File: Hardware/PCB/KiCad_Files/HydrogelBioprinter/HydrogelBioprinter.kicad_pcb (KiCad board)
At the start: 2 copper layers, 50 parts, among them Q10 MMBT4403_, Q5 RFP30N06LE, Q7 RFP30N06LE, Q8 RFP30N06LE, Q9 RFP30N06LE, U1 STM32F407VGT6, U2 M24C64-WMN6TP, U3 LM5116MHX_NOPB, U5 MAX6675ISA_, U6 TMUX1208PWR, U7 SN74HC245DWR, U9 HX711

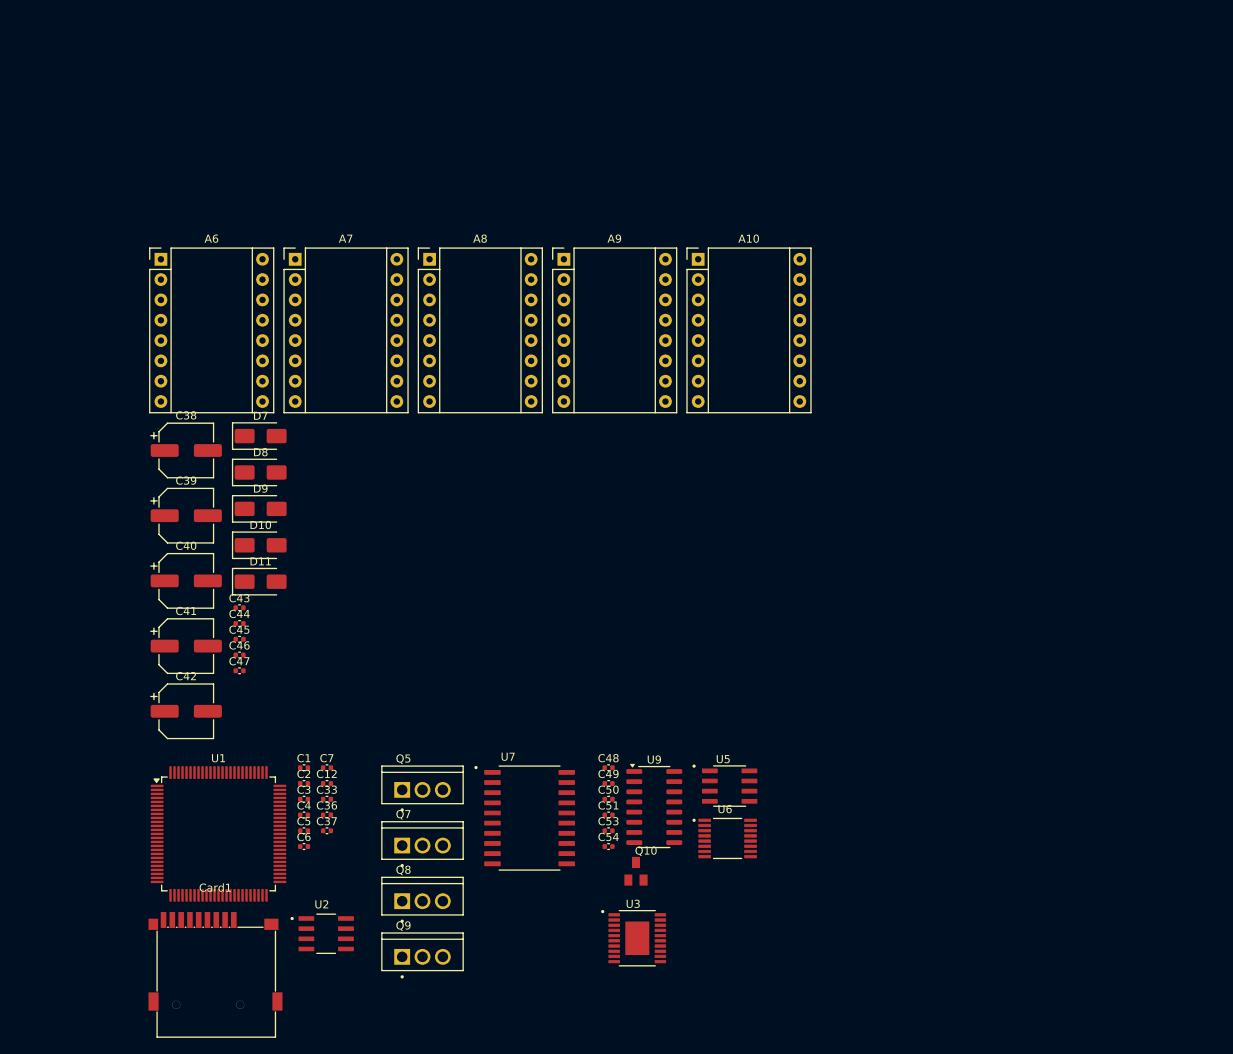
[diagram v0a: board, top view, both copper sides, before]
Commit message: Schematic Update, PCB preliminary layout, Machine Design addition, and LaTeX report addition
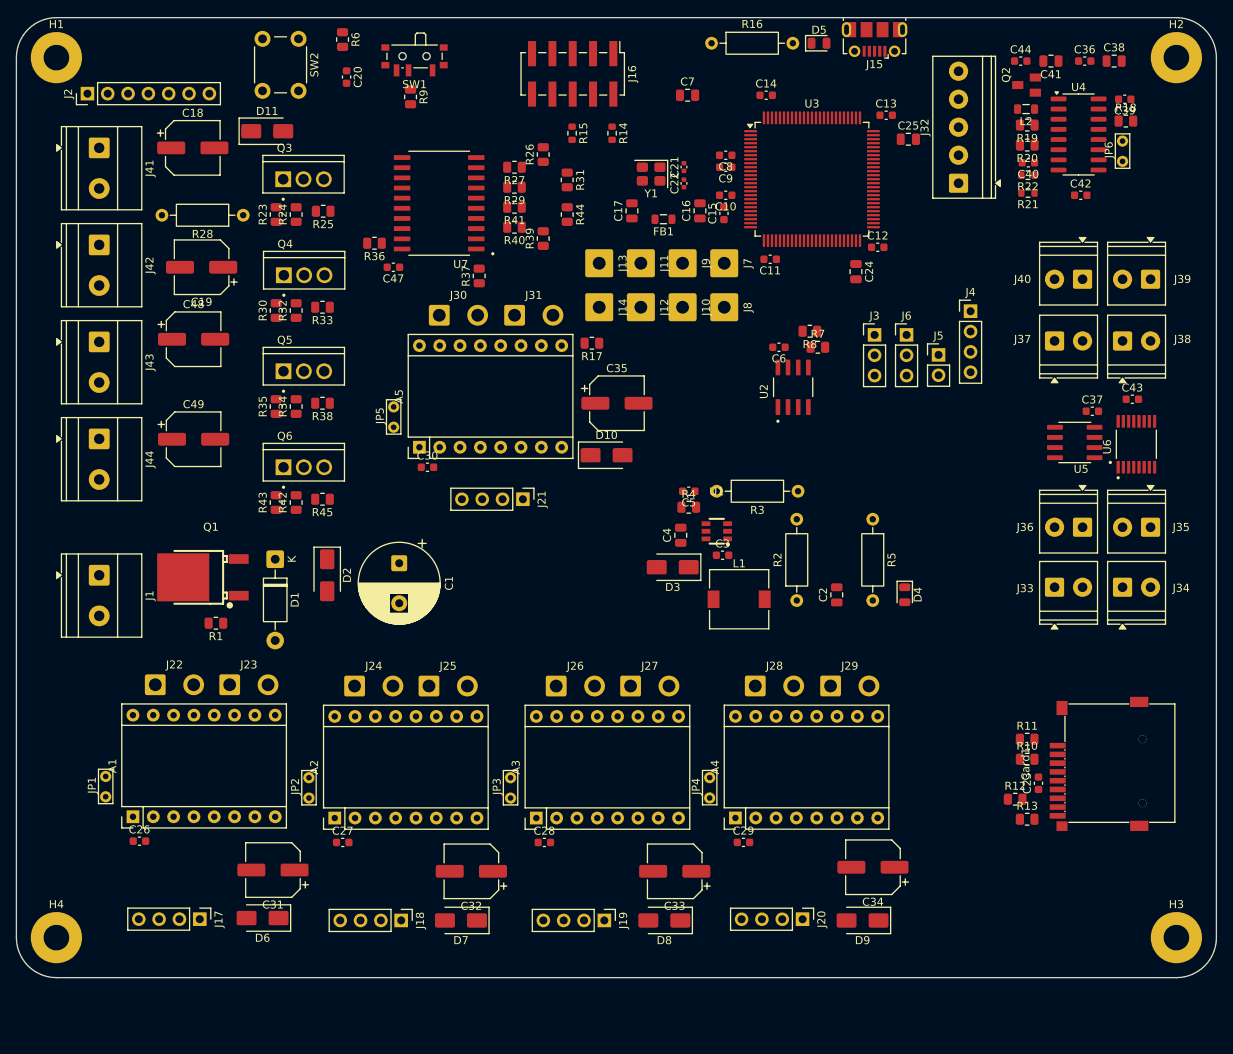
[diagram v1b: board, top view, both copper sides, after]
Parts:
- removed A10, A6, A7, A8, A9: MKS TMC2209, Module:Pololu_Breakout-16_15.2x20.3mm
- removed C45, C46, C50, C51, C53, C54: 100n, Capacitor_SMD:C_0402_1005Metric
- removed Q10: MMBT4403_, MMBT4403_:SOT23-BEC
- removed Q7, Q8, Q9: RFP30N06LE, RFP30N06LE:TRANS_RFP30N06LE
- removed U9: HX711, Package_SO:SOP-16_3.9x9.9mm_P1.27mm
- added A1: MKS TMC2209, Module:Pololu_Breakout-16_15.2x20.3mm, F.Cu at (82.6, 132.4)
- added A2: MKS TMC2209, Module:Pololu_Breakout-16_15.2x20.3mm, F.Cu at (107.8, 132.6)
- added A3: MKS TMC2209, Module:Pololu_Breakout-16_15.2x20.3mm, F.Cu at (133.0, 132.6)
- added A4: MKS TMC2209, Module:Pololu_Breakout-16_15.2x20.3mm, F.Cu at (157.9, 132.5)
- added A5: MKS TMC2209, Module:Pololu_Breakout-16_15.2x20.3mm, F.Cu at (118.4, 86.2)
- added C10: 100n, Capacitor_SMD:C_0603_1608Metric, F.Cu at (156.7, 54.7)
- added C11: 100n, Capacitor_SMD:C_0603_1608Metric, F.Cu at (162.2, 62.7)
- added C13: 100n, Capacitor_SMD:C_0603_1608Metric, F.Cu at (176.7, 44.7)
- added C14: 100n, Capacitor_SMD:C_0603_1608Metric, F.Cu at (161.7, 42.2)
- added C15: 10n, Capacitor_SMD:C_0603_1608Metric, F.Cu at (156.4, 57.0)
- added C16: 1u, Capacitor_SMD:C_0805_2012Metric, F.Cu at (153.4, 56.6)
- added C17: 1u, Capacitor_SMD:C_0805_2012Metric, F.Cu at (144.9, 56.6)
- added C18: 100u, Capacitor_SMD:CP_Elec_6.3x7.7, F.Cu at (90.0, 48.8)
- added C19: 100u, Capacitor_SMD:CP_Elec_6.3x7.7, F.Cu at (91.2, 63.7)
- added C20: 100n, Capacitor_SMD:C_0603_1608Metric, F.Cu at (109.3, 39.9)
- added C21: 10p, Capacitor_SMD:C_0402_1005Metric, F.Cu at (151.4, 51.2)
- added C22: 10p, Capacitor_SMD:C_0402_1005Metric, F.Cu at (151.4, 53.2)
- added C23: 100n, Capacitor_SMD:C_0603_1608Metric, F.Cu at (195.8, 128.2)
- added C24: 2.2uF, Capacitor_SMD:C_0805_2012Metric, F.Cu at (172.9, 64.2)
- added C25: 2.2uF, Capacitor_SMD:C_0805_2012Metric, F.Cu at (179.5, 47.7)
- added C26: 100n, Capacitor_SMD:C_0603_1608Metric, F.Cu at (83.4, 135.4)
- added C27: 100n, Capacitor_SMD:C_0603_1608Metric, F.Cu at (108.8, 135.6)
- added C28: 100n, Capacitor_SMD:C_0603_1608Metric, F.Cu at (134.0, 135.6)
- added C29: 100n, Capacitor_SMD:C_0603_1608Metric, F.Cu at (158.9, 135.6)
- added C30: 100n, Capacitor_SMD:C_0603_1608Metric, F.Cu at (119.4, 88.7)
- added C31: 100u, Capacitor_SMD:CP_Elec_6.3x7.7, F.Cu at (100.1, 139.1)
- added C32: 100u, Capacitor_SMD:CP_Elec_6.3x7.7, F.Cu at (124.9, 139.2)
- added C34: 100u, Capacitor_SMD:CP_Elec_6.3x7.7, F.Cu at (175.1, 138.7)
- added C35: 100u, Capacitor_SMD:CP_Elec_6.3x7.7, F.Cu at (143.1, 80.7)
- added C8: 100n, Capacitor_SMD:C_0603_1608Metric, F.Cu at (156.7, 49.7)
- added C9: 100n, Capacitor_SMD:C_0603_1608Metric, F.Cu at (156.7, 51.2)
- added D1: 1N4744A, Diode_THT:D_DO-41_SOD81_P10.16mm_Horizontal, F.Cu at (100.3, 100.2)
- added D2: SMAJ16A, Diode_SMD:D_SMA, F.Cu at (106.8, 102.2)
- added D3: SS34, Diode_SMD:D_SMA, F.Cu at (150.0, 101.2)
- added D4: GREEN, LED_SMD:LED_0805_2012Metric, F.Cu at (179.0, 104.6)
- added D5: BLUE, LED_SMD:LED_0805_2012Metric, F.Cu at (168.3, 35.7)
- added D6: SMAJ16A, Diode_SMD:D_SMA, F.Cu at (98.8, 145.1)
- added FB1: 120R, Inductor_SMD:L_0805_2012Metric, F.Cu at (148.9, 57.7)
- added H1: MountingHole_Pad, MountingHole:MountingHole_3.2mm_M3_Pad, F.Cu at (73.0, 37.5)
- added H2: MountingHole_Pad, MountingHole:MountingHole_3.2mm_M3_Pad, F.Cu at (213.0, 37.5)
- added H3: MountingHole_Pad, MountingHole:MountingHole_3.2mm_M3_Pad, F.Cu at (213.0, 147.5)
- added H4: MountingHole_Pad, MountingHole:MountingHole_3.2mm_M3_Pad, F.Cu at (73.0, 147.5)
- added J1: Screw_Terminal_01x02, TerminalBlock_Phoenix:TerminalBlock_Phoenix_MKDS-1,5-2-5.08_1x02_P5.08mm_Horizontal, F.Cu at (78.3, 102.2)
- added J10: Conn, Connector_Wire:SolderWire-0.75sqmm_1x01_D1.25mm_OD3.5mm, F.Cu at (151.3, 68.7)
- added J11: Conn, Connector_Wire:SolderWire-0.75sqmm_1x01_D1.25mm_OD3.5mm, F.Cu at (146.1, 63.2)
- added J12: Conn, Connector_Wire:SolderWire-0.75sqmm_1x01_D1.25mm_OD3.5mm, F.Cu at (146.1, 68.7)
- added J13: Conn, Connector_Wire:SolderWire-0.75sqmm_1x01_D1.25mm_OD3.5mm, F.Cu at (140.8, 63.2)
- added J14: Conn, Connector_Wire:SolderWire-0.75sqmm_1x01_D1.25mm_OD3.5mm, F.Cu at (140.8, 68.7)
- added J15: USB_B_Micro, Connector_USB:USB_Micro-B_Molex-105017-0001, F.Cu at (175.3, 35.2)
- added J16: Conn_02x05_Odd_Even, Connector_PinHeader_2.54mm:PinHeader_2x05_P2.54mm_Vertical_SMD, F.Cu at (137.5, 39.5)
- added J17: Conn_01x04_Pin, Connector_PinHeader_2.54mm:PinHeader_1x04_P2.54mm_Vertical, F.Cu at (90.9, 145.2)
- added J18: Conn_01x04_Pin, Connector_PinHeader_2.54mm:PinHeader_1x04_P2.54mm_Vertical, F.Cu at (116.1, 145.3)
- added J19: Conn_01x04_Pin, Connector_PinHeader_2.54mm:PinHeader_1x04_P2.54mm_Vertical, F.Cu at (141.5, 145.3)
- added J2: Conn_01x07_Pin, Connector_PinHeader_2.54mm:PinHeader_1x07_P2.54mm_Vertical, F.Cu at (76.9, 42.0)
- added J20: Conn_01x04_Pin, Connector_PinHeader_2.54mm:PinHeader_1x04_P2.54mm_Vertical, F.Cu at (166.3, 145.2)
- added J21: Conn_01x04_Pin, Connector_PinHeader_2.54mm:PinHeader_1x04_P2.54mm_Vertical, F.Cu at (131.3, 92.7)
- added J22: Conn, Connector_Wire:SolderWire-0.75sqmm_1x02_P4.8mm_D1.25mm_OD2.3mm, F.Cu at (85.4, 115.9)
- added J23: Conn, Connector_Wire:SolderWire-0.75sqmm_1x02_P4.8mm_D1.25mm_OD2.3mm, F.Cu at (94.7, 115.9)
- added J24: Conn, Connector_Wire:SolderWire-0.75sqmm_1x02_P4.8mm_D1.25mm_OD2.3mm, F.Cu at (110.3, 116.0)
- added J25: Conn, Connector_Wire:SolderWire-0.75sqmm_1x02_P4.8mm_D1.25mm_OD2.3mm, F.Cu at (119.6, 116.0)
- added J26: Conn, Connector_Wire:SolderWire-0.75sqmm_1x02_P4.8mm_D1.25mm_OD2.3mm, F.Cu at (135.5, 116.0)
- added J27: Conn, Connector_Wire:SolderWire-0.75sqmm_1x02_P4.8mm_D1.25mm_OD2.3mm, F.Cu at (144.8, 116.0)
- added J28: Conn, Connector_Wire:SolderWire-0.75sqmm_1x02_P4.8mm_D1.25mm_OD2.3mm, F.Cu at (160.4, 116.0)
- added J29: Conn, Connector_Wire:SolderWire-0.75sqmm_1x02_P4.8mm_D1.25mm_OD2.3mm, F.Cu at (169.8, 116.0)
- added J3: Conn_01x03_Pin, Connector_PinHeader_2.54mm:PinHeader_1x03_P2.54mm_Vertical, F.Cu at (175.3, 72.2)
- added J30: Conn, Connector_Wire:SolderWire-0.75sqmm_1x02_P4.8mm_D1.25mm_OD2.3mm, F.Cu at (120.9, 69.7)
- added J31: Conn, Connector_Wire:SolderWire-0.75sqmm_1x02_P4.8mm_D1.25mm_OD2.3mm, F.Cu at (130.3, 69.7)
- added J32: Screw_Terminal_01x05, TerminalBlock_Phoenix:TerminalBlock_Phoenix_PT-1,5-5-3.5-H_1x05_P3.50mm_Horizontal, F.Cu at (185.8, 53.2)
- added J33: Screw_Terminal_01x02, TerminalBlock_Phoenix:TerminalBlock_Phoenix_PT-1,5-2-3.5-H_1x02_P3.50mm_Horizontal, F.Cu at (197.8, 103.7)
- added J34: Screw_Terminal_01x02, TerminalBlock_Phoenix:TerminalBlock_Phoenix_PT-1,5-2-3.5-H_1x02_P3.50mm_Horizontal, F.Cu at (206.3, 103.7)
- added J35: Screw_Terminal_01x02, TerminalBlock_Phoenix:TerminalBlock_Phoenix_PT-1,5-2-3.5-H_1x02_P3.50mm_Horizontal, F.Cu at (209.8, 96.2)
- added J36: Screw_Terminal_01x02, TerminalBlock_Phoenix:TerminalBlock_Phoenix_PT-1,5-2-3.5-H_1x02_P3.50mm_Horizontal, F.Cu at (201.3, 96.2)
- added J37: Screw_Terminal_01x02, TerminalBlock_Phoenix:TerminalBlock_Phoenix_PT-1,5-2-3.5-H_1x02_P3.50mm_Horizontal, F.Cu at (197.8, 72.9)
- added J38: Screw_Terminal_01x02, TerminalBlock_Phoenix:TerminalBlock_Phoenix_PT-1,5-2-3.5-H_1x02_P3.50mm_Horizontal, F.Cu at (206.3, 72.9)
- added J39: Screw_Terminal_01x02, TerminalBlock_Phoenix:TerminalBlock_Phoenix_PT-1,5-2-3.5-H_1x02_P3.50mm_Horizontal, F.Cu at (209.8, 65.2)
- added J4: Conn_01x04_Pin, Connector_PinHeader_2.54mm:PinHeader_1x04_P2.54mm_Vertical, F.Cu at (187.3, 69.2)
- added J40: Screw_Terminal_01x02, TerminalBlock_Phoenix:TerminalBlock_Phoenix_PT-1,5-2-3.5-H_1x02_P3.50mm_Horizontal, F.Cu at (201.3, 65.2)
- added J41: Screw_Terminal_01x02, TerminalBlock_Phoenix:TerminalBlock_Phoenix_MKDS-1,5-2-5.08_1x02_P5.08mm_Horizontal, F.Cu at (78.3, 48.8)
- added J42: Screw_Terminal_01x02, TerminalBlock_Phoenix:TerminalBlock_Phoenix_MKDS-1,5-2-5.08_1x02_P5.08mm_Horizontal, F.Cu at (78.3, 60.9)
- added J43: Screw_Terminal_01x02, TerminalBlock_Phoenix:TerminalBlock_Phoenix_MKDS-1,5-2-5.08_1x02_P5.08mm_Horizontal, F.Cu at (78.3, 73.0)
- added J44: Screw_Terminal_01x02, TerminalBlock_Phoenix:TerminalBlock_Phoenix_MKDS-1,5-2-5.08_1x02_P5.08mm_Horizontal, F.Cu at (78.3, 85.2)
- added J5: Conn_01x02_Pin, Connector_PinHeader_2.54mm:PinHeader_1x02_P2.54mm_Vertical, F.Cu at (183.3, 74.7)
- added J6: Conn_01x03_Pin, Connector_PinHeader_2.54mm:PinHeader_1x03_P2.54mm_Vertical, F.Cu at (179.3, 72.2)
- added J7: Conn, Connector_Wire:SolderWire-0.75sqmm_1x01_D1.25mm_OD3.5mm, F.Cu at (156.5, 63.2)
- added J8: Conn, Connector_Wire:SolderWire-0.75sqmm_1x01_D1.25mm_OD3.5mm, F.Cu at (156.5, 68.7)
- added J9: Conn, Connector_Wire:SolderWire-0.75sqmm_1x01_D1.25mm_OD3.5mm, F.Cu at (151.3, 63.2)
- added JP1: Jumper_2_Bridged, TestPoint:TestPoint_Bridge_Pitch2.54mm_Drill0.7mm, F.Cu at (79.2, 127.3)
- added JP2: Jumper_2_Bridged, TestPoint:TestPoint_Bridge_Pitch2.54mm_Drill0.7mm, F.Cu at (104.6, 127.5)
- added JP3: Jumper_2_Bridged, TestPoint:TestPoint_Bridge_Pitch2.54mm_Drill0.7mm, F.Cu at (129.8, 127.5)
- added JP4: Jumper_2_Bridged, TestPoint:TestPoint_Bridge_Pitch2.54mm_Drill0.7mm, F.Cu at (154.7, 127.5)
- added JP5: Jumper_2_Bridged, TestPoint:TestPoint_Bridge_Pitch2.54mm_Drill0.7mm, F.Cu at (115.2, 81.2)
- added JP6: Jumper_2_Small_Bridged, TestPoint:TestPoint_Bridge_Pitch2.54mm_Drill0.7mm, F.Cu at (206.3, 47.9)
- added L1: 4.7u, Inductor_SMD:L_7.3x7.3_H4.5, F.Cu at (158.3, 105.2)
- added L2: 3.3uH, Inductor_SMD:L_0805_2012Metric, F.Cu at (194.2, 43.9)
- added Q1: AOD4185_C400894, AOD4185:TO-252-3_L6.6-W6.1-P4.57-LS9.9-BR-CW, F.Cu at (92.3, 102.5)
- added Q2: MMBT4403_, MMBT4403_:SOT23-BEC, F.Cu at (194.3, 40.9)
- added Q3: RFP30N06LE, RFP30N06LE:TRANS_RFP30N06LE, F.Cu at (103.9, 52.7)
- added Q4: RFP30N06LE, RFP30N06LE:TRANS_RFP30N06LE, F.Cu at (104.0, 64.7)
- added Q6: RFP30N06LE, RFP30N06LE:TRANS_RFP30N06LE, F.Cu at (103.9, 88.7)
- added R1: 100k, Resistor_SMD:R_0805_2012Metric, F.Cu at (92.9, 108.2)
- added R10: 10k, Resistor_SMD:R_0805_2012Metric, F.Cu at (194.3, 125.2)
- added R11: 10k, Resistor_SMD:R_0805_2012Metric, F.Cu at (194.3, 122.7)
- added R12: 10k, Resistor_SMD:R_0805_2012Metric, F.Cu at (192.8, 130.2)
- added R13: 10k, Resistor_SMD:R_0805_2012Metric, F.Cu at (194.3, 132.7)
- added R14: 22, Resistor_SMD:R_0603_1608Metric, F.Cu at (142.5, 47.0)
- added R15: 22, Resistor_SMD:R_0603_1608Metric, F.Cu at (137.5, 47.0)
- added R16: 470R, Resistor_THT:R_Axial_DIN0207_L6.3mm_D2.5mm_P10.16mm_Horizontal, F.Cu at (154.9, 35.7)
- added R17: 100k, Resistor_SMD:R_0805_2012Metric, F.Cu at (139.9, 73.2)
- added R18: 10k, Resistor_SMD:R_0805_2012Metric, F.Cu at (206.7, 45.4)
- added R19: 20k, Resistor_SMD:R_0805_2012Metric, F.Cu at (194.4, 45.9)
- added R2: 49.9k, Resistor_THT:R_Axial_DIN0207_L6.3mm_D2.5mm_P10.16mm_Horizontal, F.Cu at (165.5, 105.4)
- added R20: 8.2k, Resistor_SMD:R_0805_2012Metric, F.Cu at (194.4, 48.4)
- added R21: 100R, Resistor_SMD:R_0603_1608Metric, F.Cu at (194.4, 54.4)
- added R22: 100R, Resistor_SMD:R_0603_1608Metric, F.Cu at (194.4, 52.2)
- added R23: 47R, Resistor_SMD:R_0805_2012Metric, F.Cu at (100.5, 57.1)
- added R24: 47R, Resistor_SMD:R_0805_2012Metric, F.Cu at (103.0, 57.1)
- added R25: 100k, Resistor_SMD:R_0805_2012Metric, F.Cu at (106.3, 56.7)
- added R26: 100k, Resistor_SMD:R_0805_2012Metric, F.Cu at (133.8, 49.6)
- added R27: 47R, Resistor_SMD:R_0805_2012Metric, F.Cu at (130.3, 51.2)
- added R28: R, Resistor_THT:R_Axial_DIN0207_L6.3mm_D2.5mm_P10.16mm_Horizontal, F.Cu at (96.3, 57.2)
- added R29: 47R, Resistor_SMD:R_0805_2012Metric, F.Cu at (130.3, 53.7)
- added R3: 16.3k, Resistor_THT:R_Axial_DIN0207_L6.3mm_D2.5mm_P10.16mm_Horizontal, F.Cu at (165.7, 91.7)
- added R30: 47R, Resistor_SMD:R_0805_2012Metric, F.Cu at (100.5, 69.1)
- added R31: 100k, Resistor_SMD:R_0805_2012Metric, F.Cu at (136.8, 52.8)
- added R32: 47R, Resistor_SMD:R_0805_2012Metric, F.Cu at (103.0, 69.1)
- added R33: 100k, Resistor_SMD:R_0805_2012Metric, F.Cu at (106.3, 68.7)
- added R34: 47R, Resistor_SMD:R_0805_2012Metric, F.Cu at (103.0, 81.1)
- added R35: 47R, Resistor_SMD:R_0805_2012Metric, F.Cu at (100.5, 81.1)
- added R36: 10k, Resistor_SMD:R_0805_2012Metric, F.Cu at (112.8, 60.7)
- added R37: 10k, Resistor_SMD:R_0805_2012Metric, F.Cu at (125.8, 64.8)
- added R38: 100k, Resistor_SMD:R_0805_2012Metric, F.Cu at (106.3, 80.7)
- added R39: 100k, Resistor_SMD:R_0805_2012Metric, F.Cu at (133.8, 60.1)
- added R4: 10k, Resistor_SMD:R_0805_2012Metric, F.Cu at (152.0, 93.7)
- added R40: 47R, Resistor_SMD:R_0805_2012Metric, F.Cu at (130.3, 58.7)
- added R41: 47R, Resistor_SMD:R_0805_2012Metric, F.Cu at (130.3, 56.2)
- added R42: 47R, Resistor_SMD:R_0805_2012Metric, F.Cu at (103.0, 93.1)
- added R43: 47R, Resistor_SMD:R_0805_2012Metric, F.Cu at (100.5, 93.1)
- added R44: 100k, Resistor_SMD:R_0805_2012Metric, F.Cu at (136.8, 57.1)
- added R45: 100k, Resistor_SMD:R_0805_2012Metric, F.Cu at (106.3, 92.7)
- added R5: 330R, Resistor_THT:R_Axial_DIN0207_L6.3mm_D2.5mm_P10.16mm_Horizontal, F.Cu at (175.0, 95.2)
- added R6: 10k, Resistor_SMD:R_0805_2012Metric, F.Cu at (108.8, 35.2)
- added R7: 4.7k, Resistor_SMD:R_0805_2012Metric, F.Cu at (168.2, 73.7)
- added R8: 4.7k, Resistor_SMD:R_0805_2012Metric, F.Cu at (167.2, 71.7)
- added R9: 10k, Resistor_SMD:R_0805_2012Metric, F.Cu at (117.3, 42.4)
- added SW1: SW_SPDT, Button_Switch_SMD:SW_SPDT_PCM12, F.Cu at (117.8, 37.7)
- added SW2: SW_Push, Button_Switch_THT:SW_PUSH_6mm, F.Cu at (103.3, 35.1)
- added U4: HX711, Package_SO:SOP-16_3.9x9.9mm_P1.27mm, F.Cu at (200.8, 47.1)
- added Y1: 16MHz, Crystal:Crystal_SMD_3225-4Pin_3.2x2.5mm, F.Cu at (147.3, 52.0)
- C1: value 100n -> 470u; footprint Capacitor_SMD:C_0402_1005Metric -> Capacitor_THT:CP_Radial_D10.0mm_P5.00mm
- C12, C36, C37, C43, C44, C47, C5, C6: footprint Capacitor_SMD:C_0402_1005Metric -> Capacitor_SMD:C_0603_1608Metric
- C2: value 100n -> 22u; footprint Capacitor_SMD:C_0402_1005Metric -> Capacitor_SMD:C_0805_2012Metric
- C3: value 100n -> 10n; footprint Capacitor_SMD:C_0402_1005Metric -> Capacitor_SMD:C_0603_1608Metric
- C33: value 10n -> 100u; footprint Capacitor_SMD:C_0402_1005Metric -> Capacitor_SMD:CP_Elec_6.3x7.7
- C38, C41: value C_Polarized -> 10u; footprint Capacitor_SMD:CP_Elec_6.3x7.7 -> Capacitor_SMD:C_0805_2012Metric
- C39, C40, C42: value C_Polarized -> 100n; footprint Capacitor_SMD:CP_Elec_6.3x7.7 -> Capacitor_SMD:C_0603_1608Metric
- C4, C7: value 100n -> 10u; footprint Capacitor_SMD:C_0402_1005Metric -> Capacitor_SMD:C_0805_2012Metric
- C48, C49: value 100n -> 100u; footprint Capacitor_SMD:C_0402_1005Metric -> Capacitor_SMD:CP_Elec_6.3x7.7
- D10, D11, D7, D8, D9: value SMAJ28A -> SMAJ16A
- U1: value STM32F407VGT6 -> AP3211KTR-G1; footprint Package_QFP:LQFP-100_14x14mm_P0.5mm -> AP3211KTR-G1:AP3211KTR-G1
- U3: value LM5116MHX_NOPB -> STM32F407VGT6; footprint LM5116MHX_NOPB:SOP65P640X110-21N -> Package_QFP:LQFP-100_14x14mm_P0.5mm
- moved C36 133.6 mm to (201.5, 37.9)
- moved C41 130.5 mm to (197.3, 37.9), turned to 180 degrees
- moved C42 129.1 mm to (201.0, 54.7)
- moved C39 128.3 mm to (206.5, 42.7), turned to 180 degrees
- moved C38 125.8 mm to (205.2, 37.9)
- moved C44 120.3 mm to (193.5, 37.9)
- moved C40 117.5 mm to (194.5, 50.6), turned to 180 degrees
- moved C43 114.6 mm to (207.5, 80.2)
- moved Card1 113.1 mm to (203.3, 125.8), turned to 90 degrees
- moved C37 109.1 mm to (202.5, 81.7)
- moved U3 97.4 mm to (167.4, 52.7)
- moved C12 96.1 mm to (175.7, 61.2)
- moved C7 95.4 mm to (151.9, 42.2)
- moved D9 91.1 mm to (173.8, 145.3), turned to 180 degrees
- moved U2 89.9 mm to (165.1, 78.7), turned to 90 degrees
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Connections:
- C1 pad 1: +3.3V -> +12V
- C12 pad 1: /NRST -> +3.3V
- C3 pad 1: +3.3V -> Net-(D3-K)
- C3 pad 2: GND -> Net-(U1-BS)
- C33 pad 1: +3.3VA -> +12V
- C38 pad 1: +24V -> GND
- C38 pad 2: GND -> +3.3V
- C39 pad 1: +24V -> GND
- C39 pad 2: GND -> +3.3V
- C4 pad 1: +3.3V -> GND
- C4 pad 2: GND -> +12V
- C40 pad 1: +24V -> Net-(U4-VBG)
- C41 pad 1: +24V -> Net-(J32-Pin_5)
- C42 pad 1: +24V -> Net-(J32-Pin_3)
- C42 pad 2: GND -> Net-(J32-Pin_2)
- C44 pad 1: GND -> Net-(J32-Pin_5)
- C44 pad 2: +3.3V -> GND
- C47 pad 1: GND -> +3.3V
- C47 pad 2: +3.3V -> GND
- C48 pad 1: GND -> +12V
- C48 pad 2: +3.3V -> GND
- C49 pad 1: GND -> +12V
- C49 pad 2: +3.3V -> GND
- C5 pad 1: +3.3V -> GND
- C5 pad 2: GND -> +12V
- C6 pad 1: +3.3V -> GND
- C6 pad 2: GND -> +3.3V
- Card1 pad 3: MOSI_SD -> SPI1_MOSI_SD
- Card1 pad 5: SCK_SD -> SPI1_SCK_SD
- Card1 pad 7: MISO_SD -> SPI1_MISO_SD
- D10 pad 1: +24V -> +12V
- D11 pad 1: +24V -> +12V
- D7 pad 1: +24V -> +12V
- D8 pad 1: +24V -> +12V
- D9 pad 1: +24V -> +12V
- U1 pad 1: unconnected-(U1-PE2-Pad1) -> Net-(U1-BS)
- U1 pad 2: unconnected-(U1-PE3-Pad2) -> GND
- U1 pad 3: unconnected-(U1-PE4-Pad3) -> Net-(U1-FB)
- U1 pad 4: unconnected-(U1-PE5-Pad4) -> Net-(U1-EN)
- U1 pad 5: unconnected-(U1-PE6-Pad5) -> +12V
- U1 pad 6: +3.3V -> Net-(D3-K)
- U2 pad 5: SDA_EEPROM -> I2C2_SDA_EEPROM
- U2 pad 6: SCL_EEPROM -> I2C2_SCL_EEPROM
- U3 pad 1: unconnected-(U3-VIN-Pad1) -> GPIO3
- U3 pad 10: unconnected-(U3-VOUT-Pad10) -> GND
- U3 pad 11: unconnected-(U3-DEMB-Pad11) -> +3.3V
- U3 pad 12: unconnected-(U3-CS-Pad12) -> /HSE_IN
- U3 pad 13: unconnected-(U3-CSG-Pad13) -> /HSE_OUT
- U3 pad 14: unconnected-(U3-PGND-Pad14) -> NRST
- U3 pad 15: unconnected-(U3-LO-Pad15) -> Net-(J7-Pin_1)
- U3 pad 16: unconnected-(U3-VCC-Pad16) -> Net-(J9-Pin_1)
- U3 pad 17: unconnected-(U3-VCCX-Pad17) -> Net-(J11-Pin_1)
- U3 pad 18: unconnected-(U3-HB-Pad18) -> Net-(J13-Pin_1)
- U3 pad 19: unconnected-(U3-HO-Pad19) -> +3.3V
- U3 pad 2: unconnected-(U3-UVLO-Pad2) -> GPIO4
- U3 pad 20: unconnected-(U3-SW-Pad20) -> GND
- U3 pad 21: unconnected-(U3-EXP-Pad21) -> +3.3VA
- U3 pad 3: unconnected-(U3-RT/SYNC-Pad3) -> GPIO5
- U3 pad 4: unconnected-(U3-EN-Pad4) -> GPIO6
- U3 pad 5: unconnected-(U3-RAMP-Pad5) -> GPIO7
- U3 pad 6: unconnected-(U3-AGND-Pad6) -> +3.3V
- U5 pad 5: SCK_T -> SPI2_SCK_T
- U5 pad 7: MISO_T -> SPI2_MISO_T
- U6 pad 1: A0 -> A0_T
- U6 pad 15: A2 -> A2_T
- U6 pad 16: A1 -> A1_T
- U7 pad 1: unconnected-(U7-DIR-Pad1) -> Net-(U7-DIR)
- U7 pad 10: unconnected-(U7-GND-Pad10) -> GND
- U7 pad 11: unconnected-(U7-B8-Pad11) -> Net-(U7-B8)
- U7 pad 12: unconnected-(U7-B7-Pad12) -> Net-(U7-B7)
- U7 pad 13: unconnected-(U7-B6-Pad13) -> Net-(U7-B6)
- U7 pad 14: unconnected-(U7-B5-Pad14) -> Net-(U7-B5)
- U7 pad 15: unconnected-(U7-B4-Pad15) -> Net-(U7-B4)
- U7 pad 16: unconnected-(U7-B3-Pad16) -> Net-(U7-B3)
- U7 pad 17: unconnected-(U7-B2-Pad17) -> Net-(U7-B2)
- U7 pad 18: unconnected-(U7-B1-Pad18) -> Net-(U7-B1)
- U7 pad 19: unconnected-(U7-~{OE}-Pad19) -> Net-(U7-~{OE})
- U7 pad 2: unconnected-(U7-A1-Pad2) -> Net-(U7-A1)
- U7 pad 20: unconnected-(U7-VCC-Pad20) -> +3.3V
- U7 pad 3: unconnected-(U7-A2-Pad3) -> Net-(U7-A1)
- U7 pad 4: unconnected-(U7-A3-Pad4) -> Net-(U7-A3)
- U7 pad 5: unconnected-(U7-A4-Pad5) -> Net-(U7-A3)
- U7 pad 6: unconnected-(U7-A5-Pad6) -> Net-(U7-A5)
- U7 pad 7: unconnected-(U7-A6-Pad7) -> Net-(U7-A5)
- U7 pad 8: unconnected-(U7-A7-Pad8) -> Net-(U7-A7)
- U7 pad 9: unconnected-(U7-A8-Pad9) -> Net-(U7-A7)
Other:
- board outline added: 150 x 120 mm
